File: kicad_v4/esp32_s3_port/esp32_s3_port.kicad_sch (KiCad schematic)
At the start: 50 parts, among them J1 AudioJack4, J2 AudioJack4, SW1 KS33_SW_HS, SW10 KS33_SW_HS, SW11 KS33_SW_HS, SW12 KS33_SW_HS, SW13 KS33_SW_HS, SW14 KS33_SW_HS, SW15 KS33_SW_HS, SW16 KS33_SW_HS, SW17 KS33_SW_HS, SW18 KS33_SW_HS, SW19 KS33_SW_HS, SW2 KS33_SW_HS, SW20 KS33_SW_HS, SW21 KS33_SW_HS, SW3 KS33_SW_HS, SW4 KS33_SW_HS, SW5 KS33_SW_HS, SW6 KS33_SW_HS, SW7 KS33_SW_HS, SW8 KS33_SW_HS, SW9 KS33_SW_HS, U1 TP4057, U4 SSD1306-128X64-OLED-0.96

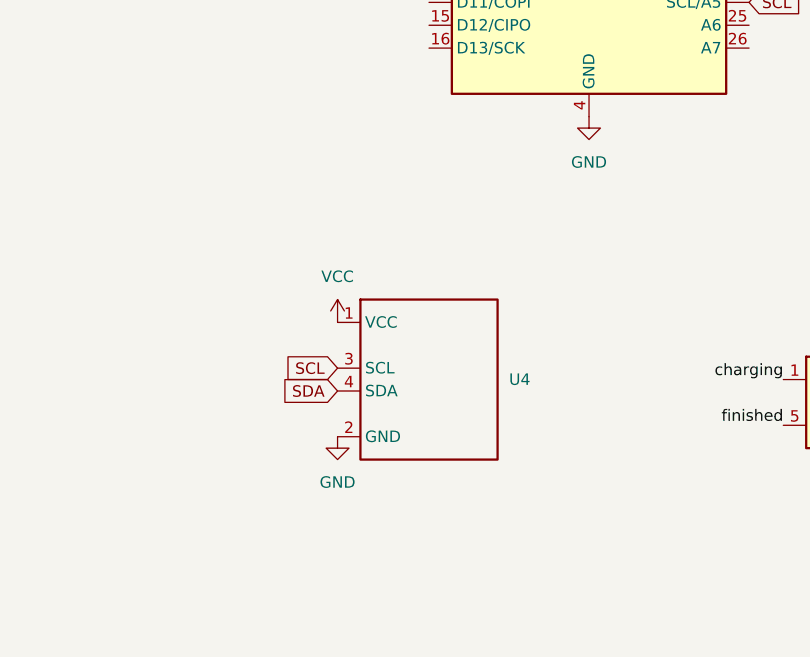
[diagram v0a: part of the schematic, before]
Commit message: ssd 1306
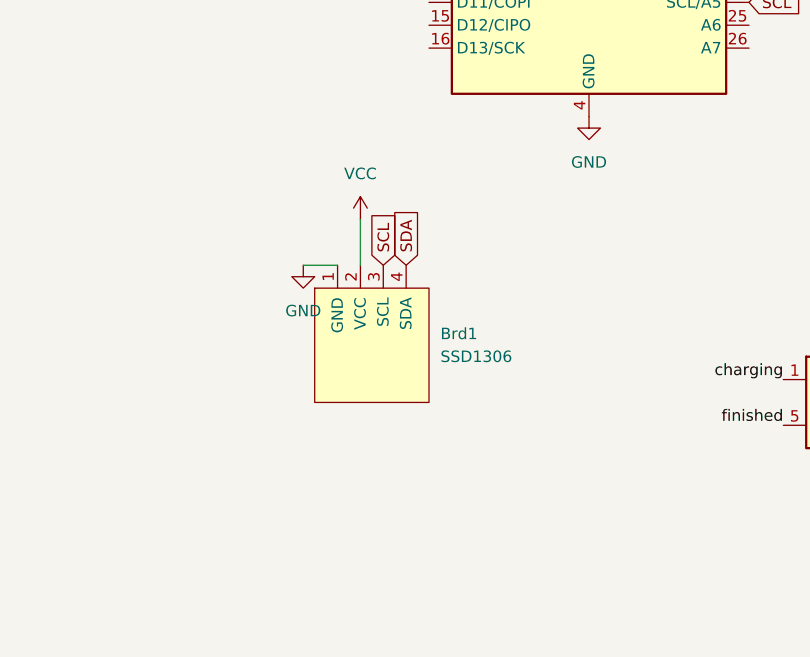
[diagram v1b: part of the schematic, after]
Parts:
- removed U4: SSD1306-128X64-OLED-0.96, Library:SSD1306, symbol Library:SSD1306-128X64-OLED-0.96
- added Brd1: SSD1306, SSD1306:128x64OLED, symbol ssd1306:SSD1306
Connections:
- net GND: now also Brd1.1 (GND)
- net SCL: now also Brd1.3 (SCL)
- net SDA: now also Brd1.4 (SDA)
- net VCC: now also Brd1.2 (VCC)
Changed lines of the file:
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@@
 	(wire
 		(pts
+			(xy 153.67 121.92) (xy 153.67 127)
+		)
+		(stroke
+			(width 0)
+			(type default)
+		)
+	)
+	(wire
+		(pts
 			(xy 52.07 160.02) (xy 52.07 179.07)
 		)
@@
 	(wire
 		(pts
+			(xy 147.32 127) (xy 151.13 127)
+		)
+		(stroke
+			(width 0)
+			(type default)
+		)
+	)
+	(wire
+		(pts
 			(xy 82.55 172.72) (xy 95.25 172.72)
 		)
@@
 		)
 	)
-	(global_label "SDA"
+	(global_label "RX"
 		(shape input)
-		(at 151.13 140.97 180)
+		(at 156.21 69.85 180)
 		(fields_autoplaced yes)
 		(effects
@@
 		)
 		(property "Intersheetrefs" "${INTERSHEET_REFS}"
-			(at 144.5767 140.97 0)
+			(at 150.7453 69.85 0)
 			(effects
 				(font
@@
 		)
 	)
-	(global_label "RX"
+	(global_label "SCL"
 		(shape input)
-		(at 156.21 69.85 180)
+		(at 156.21 127 90)
 		(fields_autoplaced yes)
 		(effects
@@
 				(size 1.27 1.27)
 			)
-			(justify right)
+			(justify left)
 		)
 		(property "Intersheetrefs" "${INTERSHEET_REFS}"
-			(at 150.7453 69.85 0)
+			(at 156.21 120.5072 90)
 			(effects
 				(font
 					(size 1.27 1.27)
 				)
-				(justify right)
+				(justify left)
 				(hide yes)
 			)
@@
 		)
 	)
-	(global_label "RX"
+	(global_label "SDA"
 		(shape input)
-		(at 106.68 86.36 0)
+		(at 158.75 127 90)
 		(fields_autoplaced yes)
 		(effects
@@
 		)
 		(property "Intersheetrefs" "${INTERSHEET_REFS}"
-			(at 112.1447 86.36 0)
+			(at 158.75 120.4467 90)
 			(effects
 				(font
@@
 		)
 	)
-	(global_label "TX"
+	(global_label "RX"
 		(shape input)
-		(at 106.68 68.58 0)
+		(at 106.68 86.36 0)
 		(fields_autoplaced yes)
 		(effects
@@
 		)
 		(property "Intersheetrefs" "${INTERSHEET_REFS}"
-			(at 111.8423 68.58 0)
+			(at 112.1447 86.36 0)
 			(effects
 				(font
@@
 		)
 	)
-	(global_label "SCL"
+	(global_label "TX"
 		(shape input)
-		(at 151.13 138.43 180)
+		(at 106.68 68.58 0)
 		(fields_autoplaced yes)
 		(effects
@@
 				(size 1.27 1.27)
 			)
-			(justify right)
+			(justify left)
 		)
 		(property "Intersheetrefs" "${INTERSHEET_REFS}"
-			(at 144.6372 138.43 0)
+			(at 111.8423 68.58 0)
 			(effects
 				(font
 					(size 1.27 1.27)
 				)
-				(justify right)
+				(justify left)
 				(hide yes)
 			)
@@
 	)
 	(symbol
-		(lib_id "Library:SSD1306-128X64-OLED-0.96")
-		(at 158.75 140.97 0)
-		(unit 1)
-		(exclude_from_sim no)
-		(in_bom yes)
-		(on_board yes)
-		(dnp no)
-		(fields_autoplaced yes)
-		(property "Reference" "U4"
-			(at 170.18 139.6999 0)
-			(effects
-				(font
-					(size 1.27 1.27)
-				)
-				(justify left)
-			)
-		)
-		(property "Value" "SSD1306-128X64-OLED-0.96"
-			(at 162.052 151.892 0)
-			(effects
-				(font
-					(size 1.27 1.27)
-				)
-				(hide yes)
-			)
-		)
-		(property "Footprint" "Library:SSD1306"
-			(at 160.782 128.778 0)
-			(effects
-				(font
-					(size 1.27 1.27)
-				)
-				(hide yes)
-			)
-		)
-		(property "Datasheet" ""
-			(at 158.75 140.97 0)
-			(effects
-				(font
-					(size 1.27 1.27)
-				)
-				(hide yes)
-			)
-		)
-		(property "Description" ""
-			(at 158.75 140.97 0)
-			(effects
-				(font
-					(size 1.27 1.27)
-				)
-				(hide yes)
-			)
-		)
-		(pin "2"
-		)
-		(pin "1"
-		)
-		(pin "3"
-		)
-		(pin "4"
-		)
-		(instances
-			(project "esp32_s3_port"
-				(path "/b35913c0-3727-49b0-a8b1-477815153830"
-					(reference "U4")
-					(unit 1)
-				)
-			)
-		)
-	)
-	(symbol
 		(lib_id "Device:Battery_Cell")
 		(at 236.22 144.78 0)
@@
 	(symbol
 		(lib_id "power:GND")
-		(at 151.13 146.05 0)
+		(at 147.32 127 0)
 		(unit 1)
 		(exclude_from_sim no)
@@
 		(fields_autoplaced yes)
 		(property "Reference" "#PWR016"
-			(at 151.13 152.4 0)
+			(at 147.32 133.35 0)
 			(effects
 				(font
@@
 		)
 		(property "Value" "GND"
-			(at 151.13 151.13 0)
+			(at 147.32 132.08 0)
 			(effects
 				(font
@@
 		)
 		(property "Footprint" ""
-			(at 151.13 146.05 0)
+			(at 147.32 127 0)
 			(effects
 				(font
@@
 		)
 		(property "Datasheet" ""
-			(at 151.13 146.05 0)
+			(at 147.32 127 0)
 			(effects
 				(font
@@
 		)
 		(property "Description" "Power symbol creates a global label with name \"GND\" , ground"
-			(at 151.13 146.05 0)
+			(at 147.32 127 0)
 			(effects
 				(font
@@
 	(symbol
 		(lib_id "power:VCC")
-		(at 151.13 133.35 0)
+		(at 153.67 121.92 0)
 		(unit 1)
 		(exclude_from_sim no)
@@
 		(fields_autoplaced yes)
 		(property "Reference" "#PWR05"
-			(at 151.13 137.16 0)
+			(at 153.67 125.73 0)
 			(effects
 				(font
@@
 		)
 		(property "Value" "VCC"
-			(at 151.13 128.27 0)
+			(at 153.67 116.84 0)
 			(effects
 				(font
@@
 		)
 		(property "Footprint" ""
-			(at 151.13 133.35 0)
+			(at 153.67 121.92 0)
 			(effects
 				(font
@@
 		)
 		(property "Datasheet" ""
-			(at 151.13 133.35 0)
+			(at 153.67 121.92 0)
 			(effects
 				(font
@@
 		)
 		(property "Description" "Power symbol creates a global label with name \"VCC\""
-			(at 151.13 133.35 0)
+			(at 153.67 121.92 0)
 			(effects
 				(font
@@
 					(unit 1)
 				)
+			)
+		)
+	)
+	(symbol
+		(lib_id "ssd1306:SSD1306")
+		(at 154.94 135.89 0)
+		(unit 1)
+		(exclude_from_sim no)
+		(in_bom yes)
+		(on_board yes)
+		(dnp no)
+		(fields_autoplaced yes)
+		(property "Reference" "Brd1"
+			(at 162.56 134.6199 0)
+			(effects
+				(font
+					(size 1.27 1.27)
+				)
+				(justify left)
+			)
+		)
+		(property "Value" "SSD1306"
+			(at 162.56 137.1599 0)
+			(effects
+				(font
+					(size 1.27 1.27)
+				)
+				(justify left)
+			)
+		)
+		(property "Footprint" "SSD1306:128x64OLED"
+			(at 154.94 129.54 0)
+			(effects
+				(font
+					(size 1.27 1.27)
+				)
+				(hide yes)
+			)
+		)
+		(property "Datasheet" ""
+			(at 154.94 129.54 0)
+			(effects
+				(font
+					(size 1.27 1.27)
+				)
+				(hide yes)
+			)
+		)
+		(property "Description" "SSD1306 OLED"
+			(at 154.94 135.89 0)
+			(effects
+				(font
+					(size 1.27 1.27)
+				)
+				(hide yes)
+			)
+		)
+		(pin "3"
+		)
+		(pin "1"
+		)
+		(pin "2"
+		)
+		(pin "4"
+		)
+		(instances
+			(project ""
+				(path "/b35913c0-3727-49b0-a8b1-477815153830"
+					(reference "Brd1")
+					(unit 1)
+				)

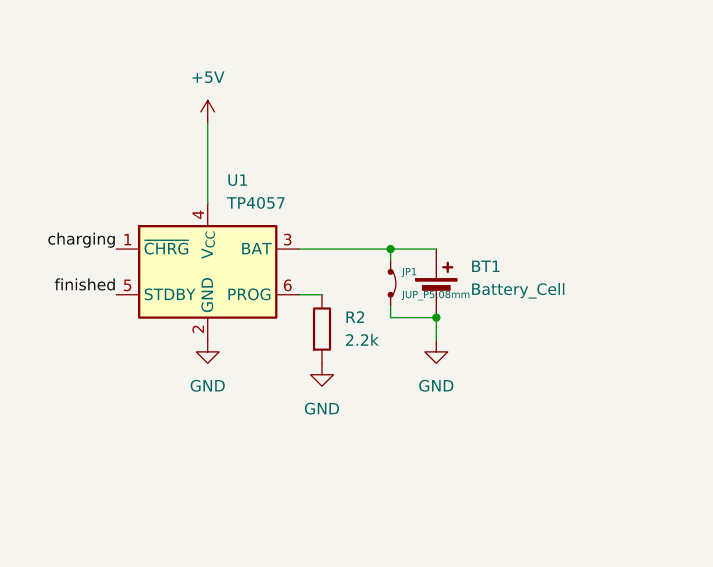
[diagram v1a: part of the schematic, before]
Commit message: battery switch
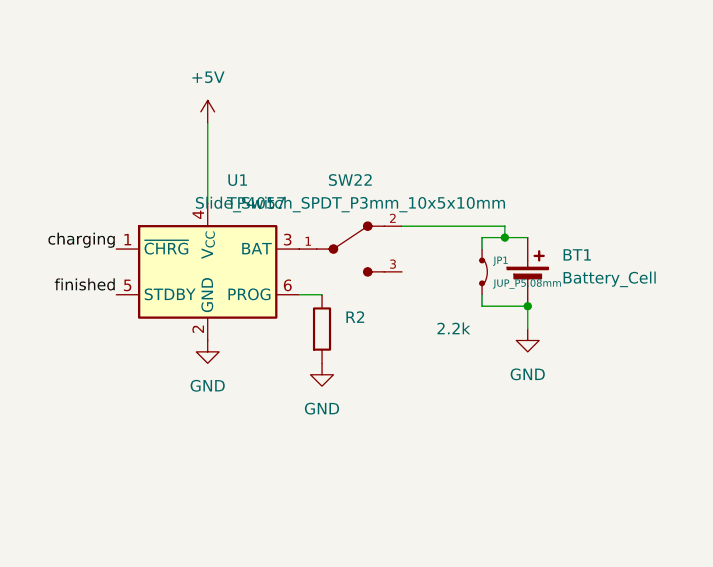
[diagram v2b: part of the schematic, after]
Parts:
- added SW22: Slide_Switch_SPDT_P3mm_10x5x10mm, PCM_SL_Devices:Slide_Switch_SPDT_P3mm_10x5x10mm, symbol PCM_SL_Devices:Slide_Switch_SPDT_P3mm_10x5x10mm
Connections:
- net at BT1.1 (+), JP1.1: now also SW22.2; no longer U1.3 (BAT)
- new net: SW22.1, U1.3 (BAT)
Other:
- moved on the sheet: BT1, JP1
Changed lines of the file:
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@@
 	)
 	(junction
-		(at 231.14 139.7)
-		(diameter 0)
-		(color 0 0 0 0)
-	)
-	(junction
 		(at 44.45 172.72)
 		(diameter 0)
@@
 	)
 	(junction
+		(at 243.84 138.43)
+		(diameter 0)
+		(color 0 0 0 0)
+	)
+	(junction
 		(at 69.85 137.16)
 		(diameter 0)
@@
 	)
 	(junction
-		(at 236.22 147.32)
+		(at 246.38 146.05)
 		(diameter 0)
 		(color 0 0 0 0)
@@
 	(wire
 		(pts
+			(xy 243.84 137.16) (xy 243.84 138.43)
+		)
+		(stroke
+			(width 0)
+			(type default)
+		)
+	)
+	(wire
+		(pts
 			(xy 26.67 140.97) (xy 26.67 160.02)
 		)
@@
 	(wire
 		(pts
+			(xy 243.84 138.43) (xy 246.38 138.43)
+		)
+		(stroke
+			(width 0)
+			(type default)
+		)
+	)
+	(wire
+		(pts
 			(xy 156.21 72.39) (xy 161.29 72.39)
 		)
@@
 	(wire
 		(pts
-			(xy 231.14 139.7) (xy 236.22 139.7)
+			(xy 241.3 138.43) (xy 243.84 138.43)
 		)
 		(stroke
@@
 	(wire
 		(pts
-			(xy 220.98 139.7) (xy 231.14 139.7)
+			(xy 69.85 153.67) (xy 82.55 153.67)
 		)
 		(stroke
@@
 	(wire
 		(pts
-			(xy 69.85 153.67) (xy 82.55 153.67)
+			(xy 31.75 172.72) (xy 44.45 172.72)
 		)
 		(stroke
@@
 	(wire
 		(pts
-			(xy 31.75 172.72) (xy 44.45 172.72)
+			(xy 52.07 115.57) (xy 52.07 124.46)
 		)
 		(stroke
@@
 	(wire
 		(pts
-			(xy 52.07 115.57) (xy 52.07 124.46)
+			(xy 39.37 114.3) (xy 39.37 124.46)
 		)
 		(stroke
@@
 	(wire
 		(pts
-			(xy 39.37 114.3) (xy 39.37 124.46)
+			(xy 69.85 137.16) (xy 82.55 137.16)
 		)
 		(stroke
@@
 	(wire
 		(pts
-			(xy 69.85 137.16) (xy 82.55 137.16)
+			(xy 64.77 124.46) (xy 64.77 140.97)
 		)
 		(stroke
@@
 	(wire
 		(pts
-			(xy 64.77 124.46) (xy 64.77 140.97)
+			(xy 232.41 137.16) (xy 243.84 137.16)
 		)
 		(stroke
@@
 	(wire
 		(pts
-			(xy 231.14 147.32) (xy 231.14 146.05)
+			(xy 241.3 146.05) (xy 241.3 144.78)
 		)
 		(stroke
@@
 	(wire
 		(pts
-			(xy 231.14 139.7) (xy 231.14 140.97)
+			(xy 241.3 138.43) (xy 241.3 139.7)
 		)
 		(stroke
@@
 	(wire
 		(pts
-			(xy 236.22 149.86) (xy 236.22 147.32)
+			(xy 246.38 148.59) (xy 246.38 146.05)
 		)
 		(stroke
@@
 	(wire
 		(pts
-			(xy 231.14 147.32) (xy 236.22 147.32)
+			(xy 241.3 146.05) (xy 246.38 146.05)
 		)
 		(stroke
@@
 	(symbol
 		(lib_id "power:GND")
-		(at 236.22 149.86 0)
+		(at 246.38 148.59 0)
 		(unit 1)
 		(exclude_from_sim no)
@@
 		(fields_autoplaced yes)
 		(property "Reference" "#PWR02"
-			(at 236.22 156.21 0)
+			(at 246.38 154.94 0)
 			(effects
 				(font
@@
 		)
 		(property "Value" "GND"
-			(at 236.22 154.94 0)
+			(at 246.38 153.67 0)
 			(effects
 				(font
@@
 		)
 		(property "Footprint" ""
-			(at 236.22 149.86 0)
+			(at 246.38 148.59 0)
 			(effects
 				(font
@@
 		)
 		(property "Datasheet" ""
-			(at 236.22 149.86 0)
+			(at 246.38 148.59 0)
 			(effects
 				(font
@@
 		)
 		(property "Description" "Power symbol creates a global label with name \"GND\" , ground"
-			(at 236.22 149.86 0)
+			(at 246.38 148.59 0)
 			(effects
 				(font
@@
 	(symbol
 		(lib_id "Device:Battery_Cell")
-		(at 236.22 144.78 0)
+		(at 246.38 143.51 0)
 		(unit 1)
 		(exclude_from_sim no)
@@
 		(fields_autoplaced yes)
 		(property "Reference" "BT1"
-			(at 240.03 141.6684 0)
+			(at 250.19 140.3984 0)
 			(effects
 				(font
@@
 		)
 		(property "Value" "Battery_Cell"
-			(at 240.03 144.2084 0)
+			(at 250.19 142.9384 0)
 			(effects
 				(font
@@
 		)
 		(property "Footprint" ""
-			(at 236.22 143.256 90)
+			(at 246.38 141.986 90)
 			(effects
 				(font
@@
 		)
 		(property "Datasheet" "~"
-			(at 236.22 143.256 90)
+			(at 246.38 141.986 90)
 			(effects
 				(font
@@
 		)
 		(property "Description" "Single-cell battery"
-			(at 236.22 144.78 0)
+			(at 246.38 143.51 0)
 			(effects
 				(font
@@
 		(on_board yes)
 		(dnp no)
-		(fields_autoplaced yes)
 		(property "Reference" "R2"
 			(at 226.06 147.3199 90)
@@
 		)
 		(property "Value" "2.2k"
-			(at 226.06 149.8599 90)
+			(at 236.22 148.5899 90)
 			(effects
 				(font
@@
 	(symbol
 		(lib_id "PCM_SL_Jumpers_THT:JUP_P5.08mm")
-		(at 231.14 143.51 270)
+		(at 241.3 142.24 270)
 		(unit 1)
 		(exclude_from_sim no)
@@
 		(fields_autoplaced yes)
 		(property "Reference" "JP1"
-			(at 232.41 142.24 90)
+			(at 242.57 140.97 90)
 			(effects
 				(font
@@
 		)
 		(property "Value" "JUP_P5.08mm"
-			(at 232.41 144.78 90)
+			(at 242.57 143.51 90)
 			(effects
 				(font
@@
 		)
 		(property "Footprint" "PCM_SL_Jumpers:JUP_P5.08mm"
-			(at 231.14 143.51 0)
+			(at 241.3 142.24 0)
 			(effects
 				(font
@@
 		)
 		(property "Datasheet" ""
-			(at 231.14 143.51 0)
+			(at 241.3 142.24 0)
 			(effects
 				(font
@@
 		)
 		(property "Description" "Through-Hole Jumpers or wire links with a pin space of 5.08mm"
-			(at 231.14 143.51 0)
+			(at 241.3 142.24 0)
 			(effects
 				(font
@@
 					(unit 1)
 				)
+			)
+		)
+	)
+	(symbol
+		(lib_id "PCM_SL_Devices:Slide_Switch_SPDT_P3mm_10x5x10mm")
+		(at 227.33 139.7 0)
+		(unit 1)
+		(exclude_from_sim no)
+		(in_bom yes)
+		(on_board yes)
+		(dnp no)
+		(fields_autoplaced yes)
+		(property "Reference" "SW22"
+			(at 226.695 132.08 0)
+			(effects
+				(font
+					(size 1.27 1.27)
+				)
+			)
+		)
+		(property "Value" "Slide_Switch_SPDT_P3mm_10x5x10mm"
+			(at 226.695 134.62 0)
+			(effects
+				(font
+					(size 1.27 1.27)
+				)
+			)
+		)
+		(property "Footprint" "PCM_SL_Devices:Slide_Switch_SPDT_P3mm_10x5x10mm"
+			(at 228.6 147.32 0)
+			(effects
+				(font
+					(size 1.27 1.27)
+				)
+				(hide yes)
+			)
+		)
+		(property "Datasheet" ""
+			(at 226.06 133.35 0)
+			(effects
+				(font
+					(size 1.27 1.27)
+				)
+				(hide yes)
+			)
+		)
+		(property "Description" "SPDT Slide Switch with 10mm length, 5mm width and 10mm hight."
+			(at 227.33 139.7 0)
+			(effects
+				(font
+					(size 1.27 1.27)
+				)
+				(hide yes)
+			)
+		)
+		(pin "1"
+		)
+		(pin "2"
+		)
+		(pin "3"
+		)
+		(instances
+			(project ""
+				(path "/b35913c0-3727-49b0-a8b1-477815153830"
+					(reference "SW22")
+					(unit 1)
+				)
